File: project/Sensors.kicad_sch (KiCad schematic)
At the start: 19 parts, among them IC201 APDS-9306-065, IC202 BMI270, IC203 BMP581, IC204 LIS2MDLTR, IC205 BME688, Q201 DMG1013UW-7

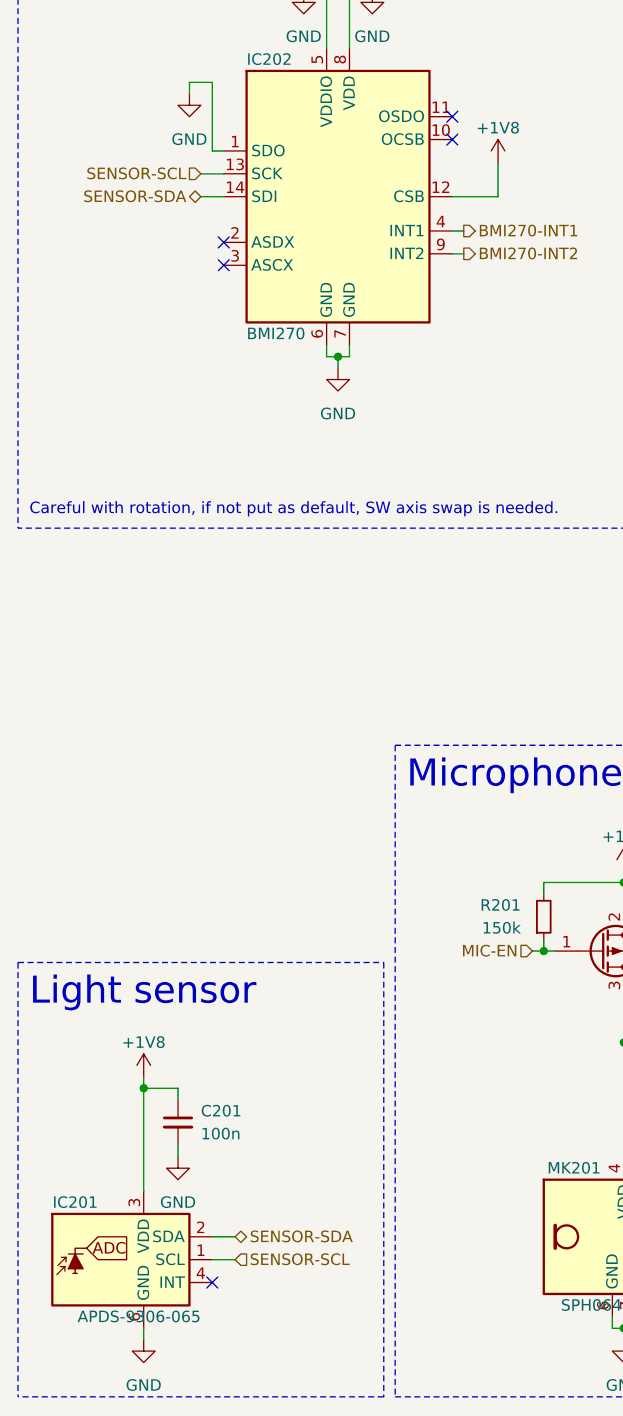
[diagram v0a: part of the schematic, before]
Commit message: Some cosmetic adjustments
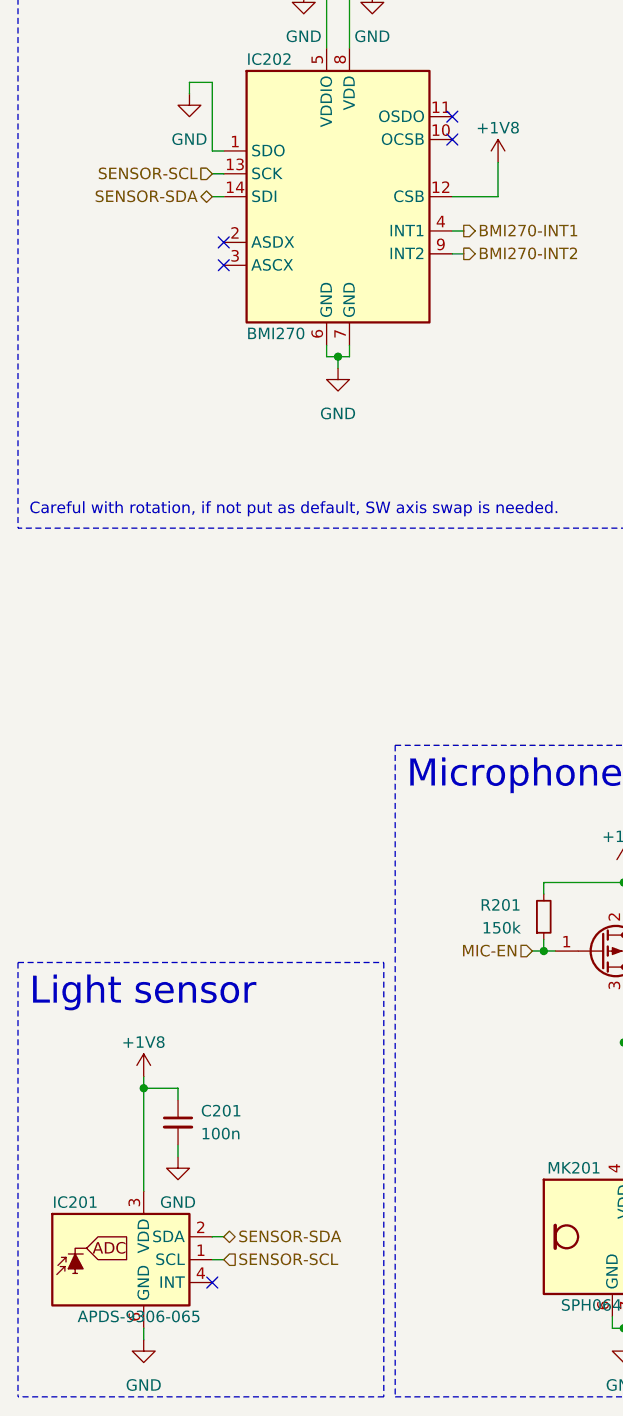
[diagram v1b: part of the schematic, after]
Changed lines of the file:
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@@
     (stroke (width 0) (type default))
   )
-  (wire (pts (xy 33.02 63.5) (xy 35.56 63.5))
+  (wire (pts (xy 34.29 63.5) (xy 35.56 63.5))
     (stroke (width 0) (type default))
   )
@@
     (stroke (width 0) (type default))
   )
-  (wire (pts (xy 34.29 181.61) (xy 36.83 181.61))
+  (wire (pts (xy 34.29 181.61) (xy 35.56 181.61))
     (stroke (width 0) (type default))
   )
@@
     (stroke (width 0) (type default))
   )
-  (wire (pts (xy 34.29 179.07) (xy 36.83 179.07))
+  (wire (pts (xy 34.29 179.07) (xy 35.56 179.07))
     (stroke (width 0) (type default))
   )
@@
     (stroke (width 0) (type default))
   )
-  (wire (pts (xy 33.02 60.96) (xy 35.56 60.96))
+  (wire (pts (xy 34.29 60.96) (xy 35.56 60.96))
     (stroke (width 0) (type default))
   )
@@
     (effects (font (size 1.27 1.27)) (justify right))
   )
-  (hierarchical_label "SENSOR-SCL" (shape input) (at 36.83 181.61 0) (fields_autoplaced)
+  (hierarchical_label "SENSOR-SCL" (shape input) (at 35.56 181.61 0) (fields_autoplaced)
     (effects (font (size 1.27 1.27)) (justify left))
   )
@@
     (effects (font (size 1.27 1.27)) (justify left))
   )
-  (hierarchical_label "SENSOR-SDA" (shape bidirectional) (at 33.02 63.5 180) (fields_autoplaced)
+  (hierarchical_label "SENSOR-SDA" (shape bidirectional) (at 34.29 63.5 180) (fields_autoplaced)
     (effects (font (size 1.27 1.27)) (justify right))
   )
@@
     (effects (font (size 1.27 1.27)) (justify left))
   )
-  (hierarchical_label "SENSOR-SCL" (shape input) (at 33.02 60.96 180) (fields_autoplaced)
-    (effects (font (size 1.27 1.27)) (justify right))
-  )
-  (hierarchical_label "SENSOR-SDA" (shape bidirectional) (at 36.83 179.07 0) (fields_autoplaced)
-    (effects (font (size 1.27 1.27)) (justify left))
-  )
+  (hierarchical_label "SENSOR-SCL" (shape input) (at 34.29 60.96 180) (fields_autoplaced)
+    (effects (font (size 1.27 1.27)) (justify right))
+  )
+  (hierarchical_label "SENSOR-SDA" (shape bidirectional) (at 35.56 179.07 0) (fields_autoplaced)
+    (effects (font (size 1.27 1.27)) (justify left))
+  )
